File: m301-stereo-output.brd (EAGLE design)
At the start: 100 x 50 mm, 89 parts, among them U1 ERM1-5MM, U4 G3VM-62C1, U5 FX2-20P-1.27DS, U6 FX2-20S-1.27DS, U7 ERM1-5MM

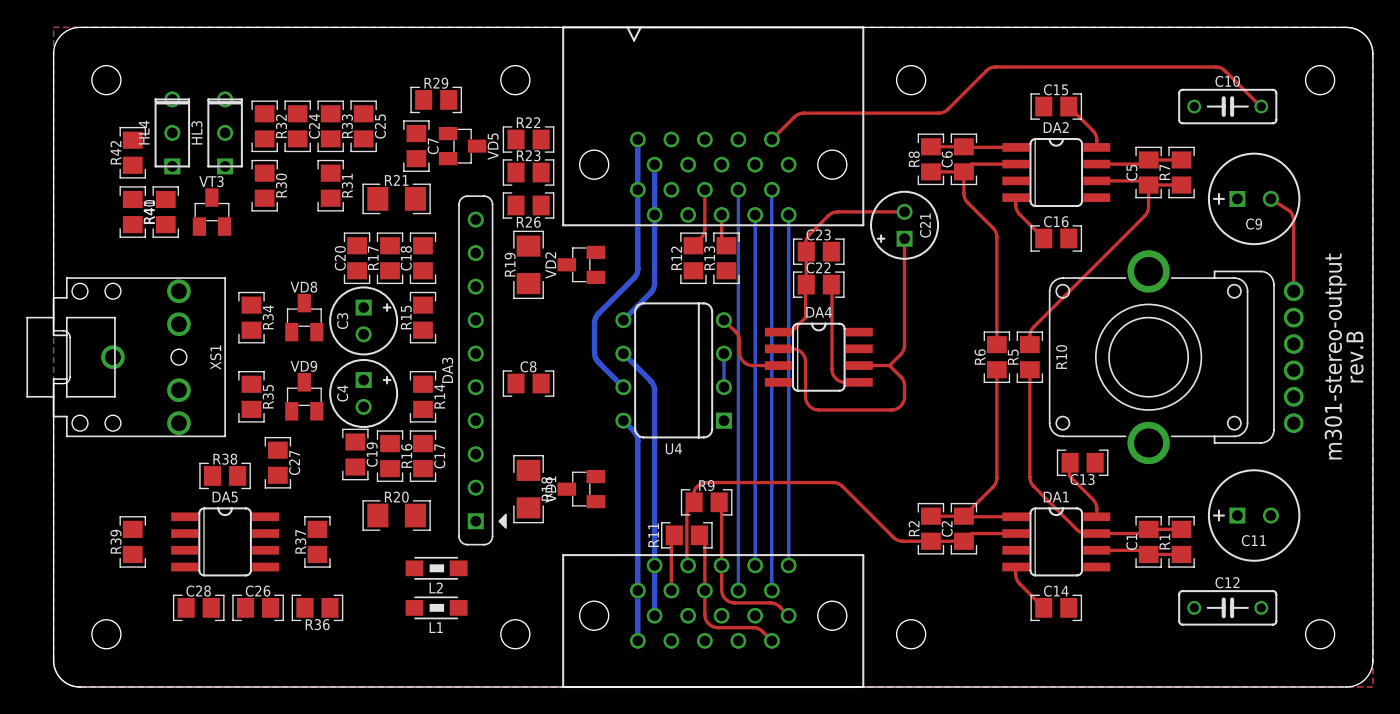
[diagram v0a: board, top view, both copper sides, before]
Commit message: M301 Update
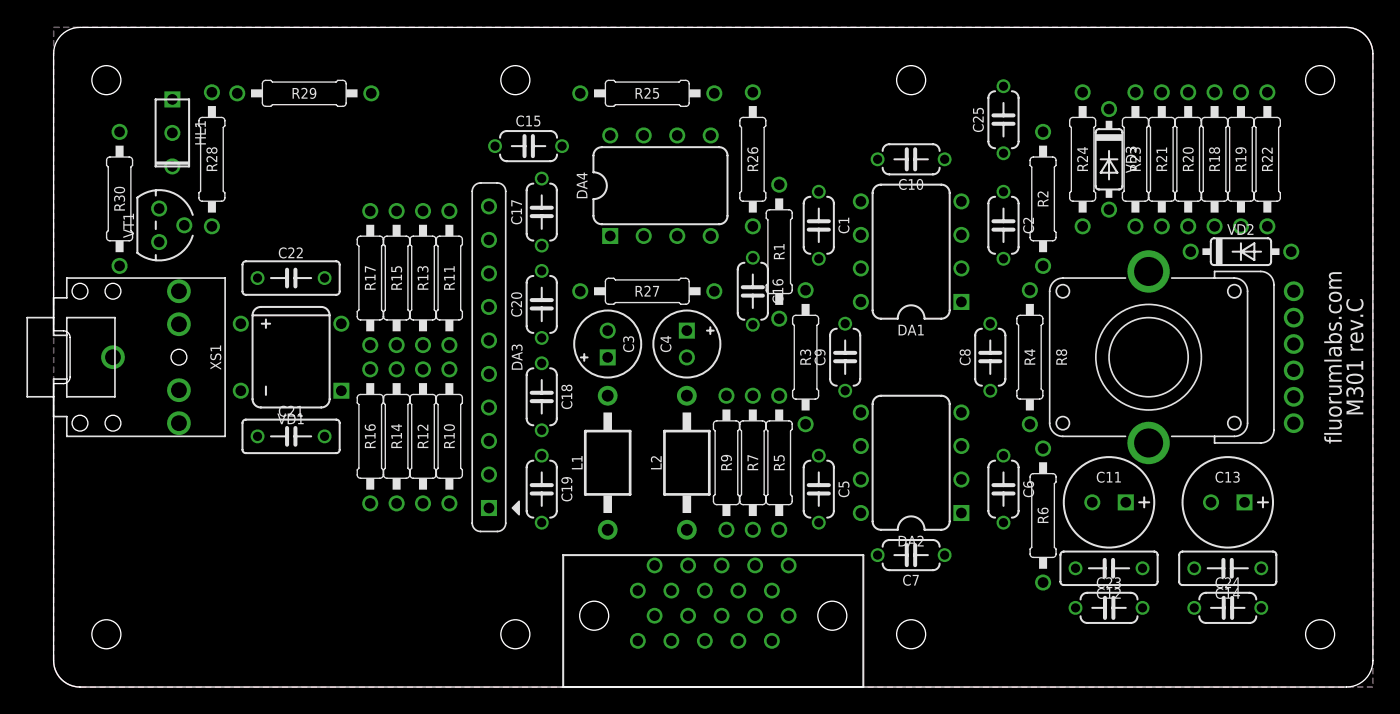
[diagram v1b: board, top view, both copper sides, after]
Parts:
- removed C26, C27, C28: 100N, capacitors:C-0805
- removed DA5: LM2903M, ic-fairchild:SO-8
- removed HL3: RED/BLUE(2MMX5MM,CC), optoelectronics:LED2X5-3PIN
- removed O3: 450-CP156(15MM,BLACK/WHITE), hardware:EMPTY
- removed R31: 10M, resistors:R-0805
- removed R32, R33: 100K, resistors:R-0805
- removed R34, R35: 47K, resistors:R-0805
- removed R36: 330K, resistors:R-0805
- removed R37: 22K, resistors:R-0805
- removed R38: 4K7, resistors:R-0805
- removed R39: 100R, resistors:R-0805
- removed R40: 2K2, resistors:R-0805
- removed R41: 10K, resistors:R-0805
- removed R42: 1K8, resistors:R-0805
- removed U7: ERM1-5MM, hardware:EMPTY
- removed VD5, VD8, VD9: BAS16, diodes:SOT23
- removed VT3: BC848, transistors-npn:SOT23
- added R24: 330K(TH), resistors:R-0207/10
- added R25: 22K(TH), resistors:R-0207/10
- added R27: 100R(TH), resistors:R-0207/10
- added R28, R3, R4: 10K(TH), resistors:R-0207/10
- added U2: SCREW-M2X8, hardware:EMPTY
- added U3: NUT-M2-SELFLOCK, hardware:EMPTY
- added VD3: 1N4148, diodes:DO35-7
- added VT1: BC548, transistors-npn:TO92
- C1, C2, C5, C6: value 22P -> 22P(TH); device capacitors:C-0805 -> capacitors:C050-024X044
- C10: value 100N(FILM) -> 100N(TH); device capacitors:C050-025X075 -> capacitors:C050-024X044
- C13: value 100N -> 33U/25V; device capacitors:C-0805 -> capacitors-electrolytic:E2,5-7
- C14, C22: value 100N -> 100N(FILM); device capacitors:C-0805 -> capacitors:C050-025X075
- C15, C16, C23, C24, C25, C7, C8: value 100N -> 100N(TH); device capacitors:C-0805 -> capacitors:C050-024X044
- C17, C18: value 22P -> 100N(TH); device capacitors:C-0805 -> capacitors:C050-024X044
- C19, C20: value 100N -> 22P(TH); device capacitors:C-0805 -> capacitors:C050-024X044
- C21: value 10U/35V -> 100N(FILM); device capacitors-electrolytic:E2-5 -> capacitors:C050-025X075
- C9: value 33U/25V -> 100N(TH); device capacitors-electrolytic:E2,5-7 -> capacitors:C050-024X044
- DA1, DA2: value NJM2068M -> NJM2068D; device ic-jrc:SO-8 -> ic-jrc:DIP-8
- DA4: value NE555D -> LM2903N; device ic-logic:SO-8 -> ic-fairchild:DIP-8
- L1, L2: value BLM31AJ601SN1L -> BL01RN1A1F1J; device inductors:1206 -> inductors:BL01RN1A
- O1: value (none) -> 450-AA150(15MM,D,BLACK); device text:EMPTY -> hardware:EMPTY
- O2: value 450-AA150(15MM,D,BLACK) -> 450-CP156(15MM,BLACK/WHITE)
- PCB1: value rev.B -> M301 rev.C; device module-footprints:ST2-BOARD-50 -> module-footprints:ST2-BOARD-50-END
- R1, R11, R2, R5, R6, R7, R9: value 10K -> 10K(TH); device resistors:R-0805 -> resistors:R-0207/10
- R10: value 2*A10K -> 10K(TH); device potentiometers:RV11-DUAL -> resistors:R-0207/10
- R12, R13: value 100K -> 33K(TH); device resistors:R-0805 -> resistors:R-0207/10
- R14, R15: value 10K -> 10R(TH); device resistors:R-0805 -> resistors:R-0207/10
- R16, R17: value 33K -> 2R(TH); device resistors:R-0805 -> resistors:R-0207/10
- R18: value 10R(1206) -> 10M(TH); device resistors:R-1206 -> resistors:R-0207/10
- R19: value 10R(1206) -> 100K(TH); device resistors:R-1206 -> resistors:R-0207/10
- R20: value 2R(1206) -> 10M(TH); device resistors:R-1206 -> resistors:R-0207/10
- R21: value 2R(1206) -> 100K(TH); device resistors:R-1206 -> resistors:R-0207/10
- R22: value 10K -> 47K(TH); device resistors:R-0805 -> resistors:R-0207/10
- R23: value 100K -> 47K(TH); device resistors:R-0805 -> resistors:R-0207/10
- R26: value 1K5 -> 4K7(TH); device resistors:R-0805 -> resistors:R-0207/10
- R29: value 3K3 -> 2K2(TH); device resistors:R-0805 -> resistors:R-0207/10
- R30: value 10M -> 1K8(TH); device resistors:R-0805 -> resistors:R-0207/10
- R8: value 10K -> 2*A10K; device resistors:R-0805 -> potentiometers:RV11-DUAL
- U1: value ERM1-5MM -> SCREW-M2X8
- U4: value G3VM-62C1 -> NUT-M2-SELFLOCK; device optoelectronics:DIL08 -> hardware:EMPTY
- U5: value FX2-20P-1.27DS -> FX2-20S-1.27DS
- U6: value FX2-20S-1.27DS -> ERM1-5MM
- VD1: value BAV199 -> DF01M; device diodes:SOT23 -> diodes:MDIP-4
- VD2: value BAV199 -> 1N4148; device diodes:SOT23 -> diodes:DO35-7
- moved O2 274.6 mm to (95.0, -106.0)
- moved O1 270.9 mm to (92.0, -106.0)
- moved U1 214.7 mm to (98.0, -106.0)
- moved U6 143.5 mm to (13.0, -109.0)
- moved U5 141.8 mm to (10.0, -109.0)
- moved U4 138.9 mm to (7.00, -109.0), turned to 0 degrees
- moved C24 79.4 mm to (89.0, 6.00), turned to 0 degrees
- moved R20 65.8 mm to (86.0, 40.0), turned to 270 degrees
- moved R21 58.1 mm to (84.0, 40.0), turned to 90 degrees
- moved R18 57.7 mm to (88.0, 40.0)
- moved R22 56.0 mm to (92.0, 40.0), turned to 270 degrees
- moved R19 54.6 mm to (90.0, 40.0)
- moved R10 53.3 mm to (30.0, 19.0)
- moved VD2 50.0 mm to (90.0, 33.0), turned to 0 degrees
- moved C21 49.2 mm to (18.0, 19.0), turned to 0 degrees
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- renumbered HL4 to HL1
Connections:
- removed net CHAIN+15: PCB1.A+15', PCB1.B+15', R29.2, U4.7
- removed net N$2: PCB1.ARFBK', R13.2
- removed net N$27: C22.2, DA4.5
- removed net N$28: C21.+, DA4.2, DA4.6, R23.1, VD5.1
- removed net N$29: R26.2, U4.1
- removed net N$31: DA4.3, U4.4
- removed net N$36: U4.2, U4.3
- removed net N$4: PCB1.ALFBK', R12.2
- removed net N$41: PCB1.ACV1, PCB1.ACV1'
- removed net N$42: PCB1.ACV2, PCB1.ACV2'
- removed net N$44: HL3.A2, R29.1
- removed net N$51: PCB1.A-15', PCB1.B-15', U4.5
- removed net SENSE: PCB1.BSENSE', R22.2, R23.2, R26.1, VD5.2
- net +15V: now also C17.2, C9.2, DA4.8, R18.2, R20.2, R25.2, VD1.3; no longer C13.2, C27.2, DA5.8, R30.2, R31.2, R37.2, VD1.2, VD2.2
- net -15V: now also C10.1, C18.1, DA4.4, VD1.4, VT1.3; no longer C14.1, C21.-, C22.1, C23.1, C28.1, DA4.1, DA5.4, HL3.K, R22.1, VD1.1, VD2.1, VT3.2
- net GND: now also C10.2, C17.1, C18.2, C21.1, C22.1, C25.1, C9.1, R11.1, R19.1, R21.1, R24.1, R27.1, R29.2, R30.2, R8.1, R8.1'; no longer C13.1, C14.2, C19.1, C20.1, C23.2, C26.1, C27.1, C28.2, DA4.4, DA4.8, PCB1.B4', PCB1.B5', PCB1.B6', PCB1.B7', PCB1.B8', R10.1', R12.1, R13.1, R14.1, R15.1, R32.1, R33.1, R36.1, R39.1, R40.2, R42.2
- net LMIX: now also R9.1; no longer R11.1
- net N$1: no longer U4.8
- net N$10: now also C13.-, C14.2, C24.1, R8.3; no longer C11.-, C12.2, C25.1, PCB1.BOUTR', R10.3
- net N$11: now also C19.2, R12.2, R14.2, VD1.1; no longer C17.2, R18.2, R20.2, VD1.3
- net N$12: now also C19.1, R10.2, R12.1; no longer C17.1, R14.2, R16.1
- net N$13: now also R22.2, VD2.A; no longer R34.2, VD8.1
- net N$14: now also R14.1; no longer R18.1
- net N$15: now also C11.-, C12.2, C23.1, R8.3'; no longer C10.2, C24.1, C9.-, PCB1.BOUTL', R10.3'
- net N$16: now also C21.2, R16.1; no longer C19.2, R20.1
- net N$17: now also C23.2, R18.1, R19.2, R22.1; no longer C24.2, R30.1, R32.2, R34.1
- net N$18: now also C24.2, R20.1, R21.2, R23.1; no longer C25.2, R31.1, R33.2, R35.1
- net N$20: now also R23.2, VD3.A; no longer R35.2, VD9.1
- net N$21: now also C25.2, DA4.3, DA4.5, R24.2, VD2.C, VD3.C; no longer C26.2, DA5.3, DA5.5, R36.2, VD8.2, VD9.2
- net N$22: now also C20.1, R11.2, R13.1; no longer C18.1, R15.2, R17.1
- net N$23: now also DA4.2, R26.1, R27.2; no longer DA5.2, R38.1, R39.2
- net N$24: now also C20.2, R13.2, R15.2, VD1.2; no longer C18.2, R19.2, R21.2, VD2.3
- net N$25: now also DA4.1, R30.1, VT1.1; no longer DA5.1, R42.1, VT3.3
- net N$3: now also R8.2; no longer R10.2
- net N$38: no longer PCB1.ASMBDAT'
- net N$39: now also R7.2; no longer R9.2
- net N$40: now also R9.2; no longer R11.2
- net N$43: no longer PCB1.ASMBCLK'
- net N$45: now also R15.1; no longer R19.1
- net N$46: now also C22.2, R17.1; no longer C20.2, R21.1
- net N$47: now also DA4.6, R25.1, R26.2; no longer DA5.6, R37.1, R38.2
- net N$48: now also DA4.7, R28.2, R29.1; no longer DA5.7, R40.1, R41.2
- net N$49: now also R28.1, VT1.2; no longer R41.1, VT3.1
- net N$5: no longer U4.6
- net N$54: now also R3.2, R5.1; no longer R5.2, R7.1
- net N$55: now also C11.+, C12.1, R5.2; no longer C10.1, C9.+, R7.2
- net N$56: now also R4.2, R6.1; no longer R6.2, R8.1
- net N$57: now also C13.+, C14.1, R6.2; no longer C11.+, C12.1, R8.2
- net N$7: now also R3.1; no longer R5.1
- net N$8: now also R4.1; no longer R6.1
- net N$9: now also R8.2'; no longer R10.2'
- net RMIX: now also R7.1; no longer R9.1
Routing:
- net N$15: track 48.3 -> 0.00 mm
- net RMIX: track 32.3 -> 0.00 mm
- net N$41: track 30.4 -> 0.00 mm
- net N$38: track 30.4 -> 0.00 mm
- net N$28: track 28.5 -> 0.00 mm
- net N$43: track 26.6 -> 0.00 mm
- net N$42: track 26.6 -> 0.00 mm
- net -15V: track 24.6 -> 0.00 mm
- net N$54: track 22.3 -> 0.00 mm
- net N$7: track 21.7 -> 0.00 mm
- net CHAIN+15: track 20.8 -> 0.00 mm
- net N$5: track 20.8 -> 0.00 mm
- net N$56: track 20.7 -> 0.00 mm
- net N$8: track 18.5 -> 0.00 mm
- net N$1: track 17.1 -> 0.00 mm
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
